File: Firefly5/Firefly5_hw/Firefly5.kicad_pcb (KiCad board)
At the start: 2 copper layers, 63 x 16 mm, 52 parts, among them Q1 LED_5050, Q2 ALS-PT19-315C, SW1 SWITCH, SW2 Btn4x4, SW3 Btn4x4

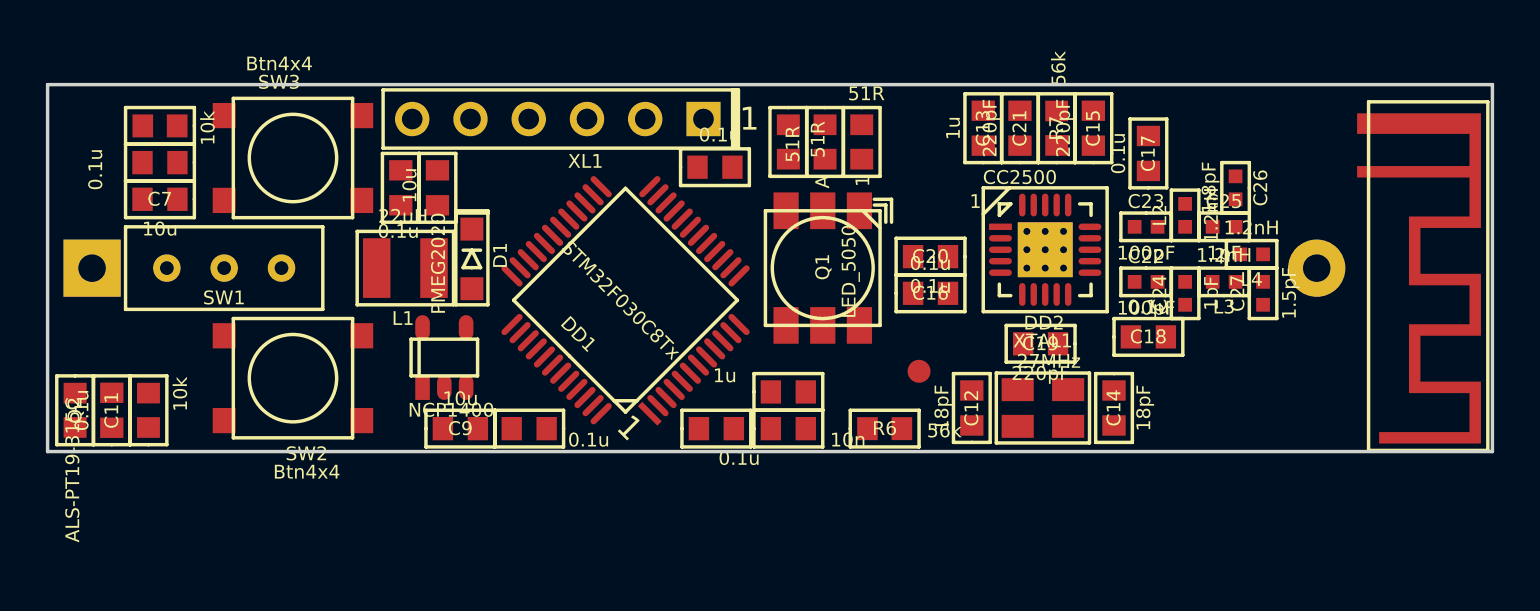
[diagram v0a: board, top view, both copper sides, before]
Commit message: Firefly5 ready for production
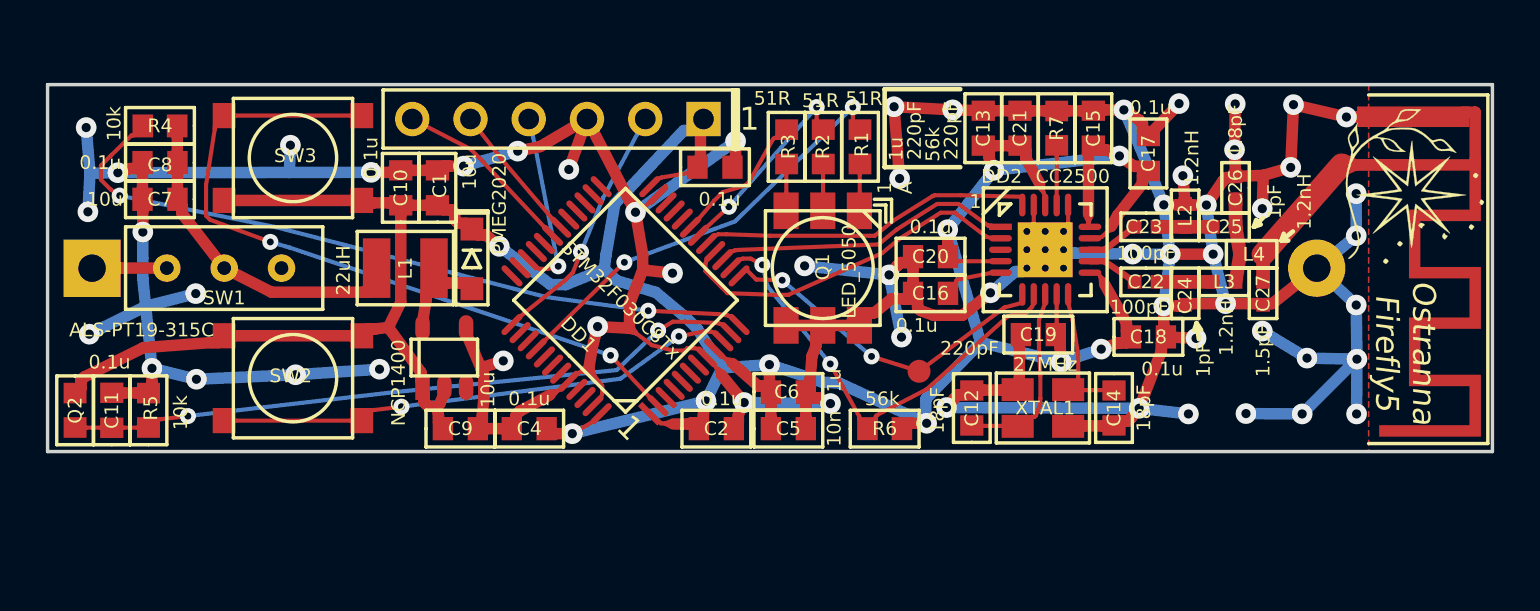
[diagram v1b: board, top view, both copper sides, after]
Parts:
- added Logo1: Logo, Pictures:Ostranna_8x8, F.Cu at (221.8, 99.9)
- moved C19 0.41 mm to (205.6, 106.0)
- moved ANT1 0.30 mm to (220.0, 98.6)
- moved R1 0.22 mm to (197.8, 97.8)
- moved R2 0.22 mm to (196.2, 97.8)
- moved R3 0.22 mm to (194.6, 97.8)
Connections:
- DA1 pad 3: (no net) -> Net-(DA1-Pad3)
- DD1 pad 20: (no net) -> Net-(DD1-Pad20)
- DD1 pad 21: (no net) -> Net-(DD1-Pad21)
- DD1 pad 22: (no net) -> Net-(DD1-Pad22)
- DD1 pad 25: (no net) -> Net-(DD1-Pad25)
- DD1 pad 26: (no net) -> Net-(DD1-Pad26)
- DD1 pad 27: (no net) -> Net-(DD1-Pad27)
- DD1 pad 28: (no net) -> Net-(DD1-Pad28)
- DD1 pad 29: (no net) -> Net-(DD1-Pad29)
- DD1 pad 3: (no net) -> Net-(DD1-Pad3)
- DD1 pad 32: (no net) -> Net-(DD1-Pad32)
- DD1 pad 33: (no net) -> Net-(DD1-Pad33)
- DD1 pad 35: (no net) -> Net-(DD1-Pad35)
- DD1 pad 36: (no net) -> Net-(DD1-Pad36)
- DD1 pad 38: (no net) -> Net-(DD1-Pad38)
- DD1 pad 39: (no net) -> Net-(DD1-Pad39)
- DD1 pad 4: (no net) -> Net-(DD1-Pad4)
- DD1 pad 41: (no net) -> Net-(DD1-Pad41)
- DD1 pad 42: (no net) -> Net-(DD1-Pad42)
- DD1 pad 43: (no net) -> Net-(DD1-Pad43)
- DD1 pad 45: (no net) -> Net-(DD1-Pad45)
- DD1 pad 46: (no net) -> Net-(DD1-Pad46)
- DD1 pad 5: (no net) -> Net-(DD1-Pad5)
- DD1 pad 6: (no net) -> Net-(DD1-Pad6)
- DD1 pad 7: (no net) -> Net-(DD1-Pad7)
- DD2 pad 3: (no net) -> Net-(DD2-Pad3)
- SW1 pad 3: (no net) -> Net-(SW1-Pad3)
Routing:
- net GND: track 0.00 -> 249.7 mm, vias 0 -> 58
- net +3.3V: track 0.00 -> 150.7 mm, vias 0 -> 10
- net /BTN2: track 0.00 -> 32.3 mm, vias 0 -> 2
- net Net-(DD1-Pad12): track 0.00 -> 32.0 mm, vias 0 -> 2
- net /LUM_MEAS: track 0.00 -> 29.8 mm, vias 0 -> 2
- net /BTN1: track 0.00 -> 22.8 mm, vias 0 -> 2
- net /CC_CS: track 0.00 -> 19.9 mm, vias 0 -> 2
- net /BLUE_LED: track 0.00 -> 18.8 mm, vias 0 -> 2
- net /CC_MISO: track 0.00 -> 15.6 mm
- net /CC_GDO0: track 0.00 -> 15.3 mm, vias 0 -> 2
- net /CC_MOSI: track 0.00 -> 14.8 mm
- net +BATT: track 0.00 -> 14.6 mm
- net /CC_SCK: track 0.00 -> 13.1 mm
- net /SWCLK: track 0.00 -> 10.9 mm, vias 0 -> 1
- net Net-(ANT1-Pad1): track 0.00 -> 10.6 mm
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- added copper zone on B.Cu, net GND
- added copper zone on F.Cu, net GND
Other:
- net class Default: trace_width 0.2 -> 0.18; via_dia 0.9 -> 0.7; via_drill 0.4 -> 0.3
- net class Wide: clearance 0.2 -> 0.18
- rule trace_min: 0.2 -> 0.1
- rule via_min_drill: 0.4 -> 0.3
- rule via_min_size: 0.889 -> 0.6
- board text added: "Ostranna Firefly5"

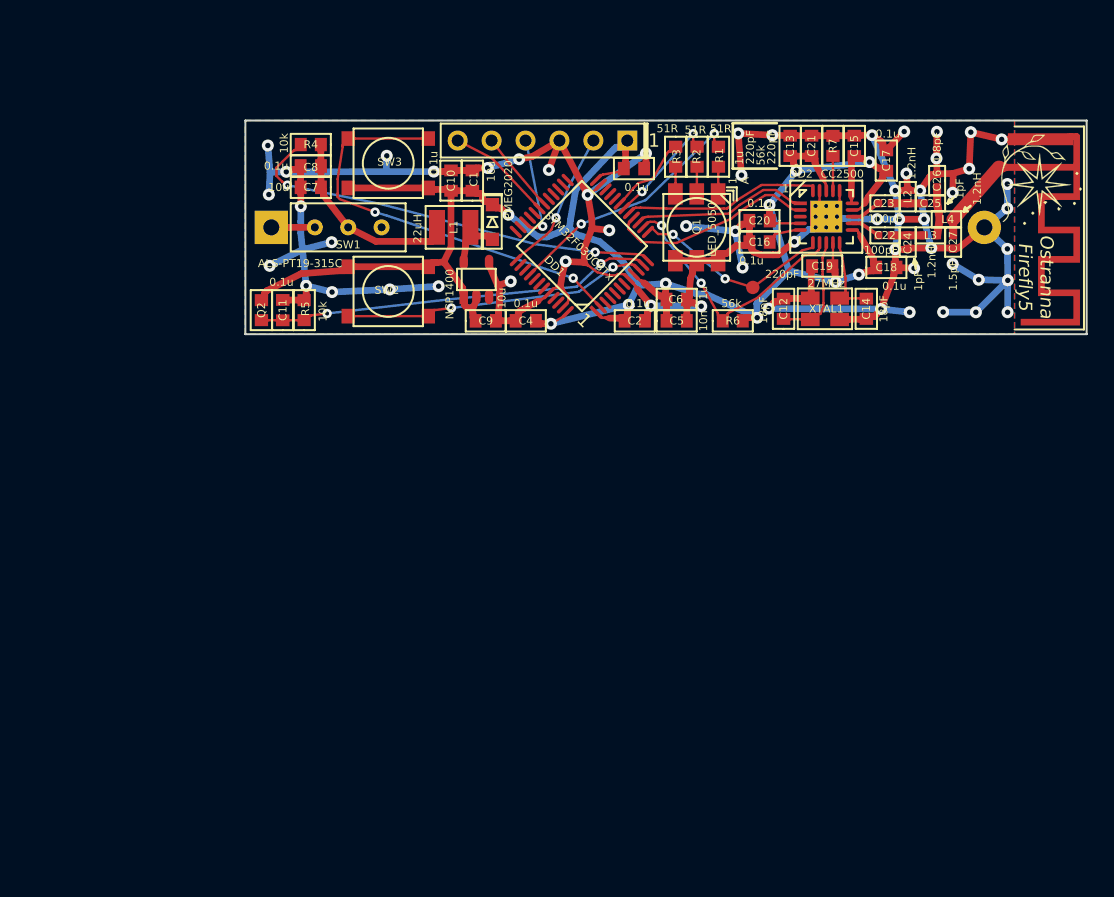
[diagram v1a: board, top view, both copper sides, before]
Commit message: * Something in FF3 + FF5.1
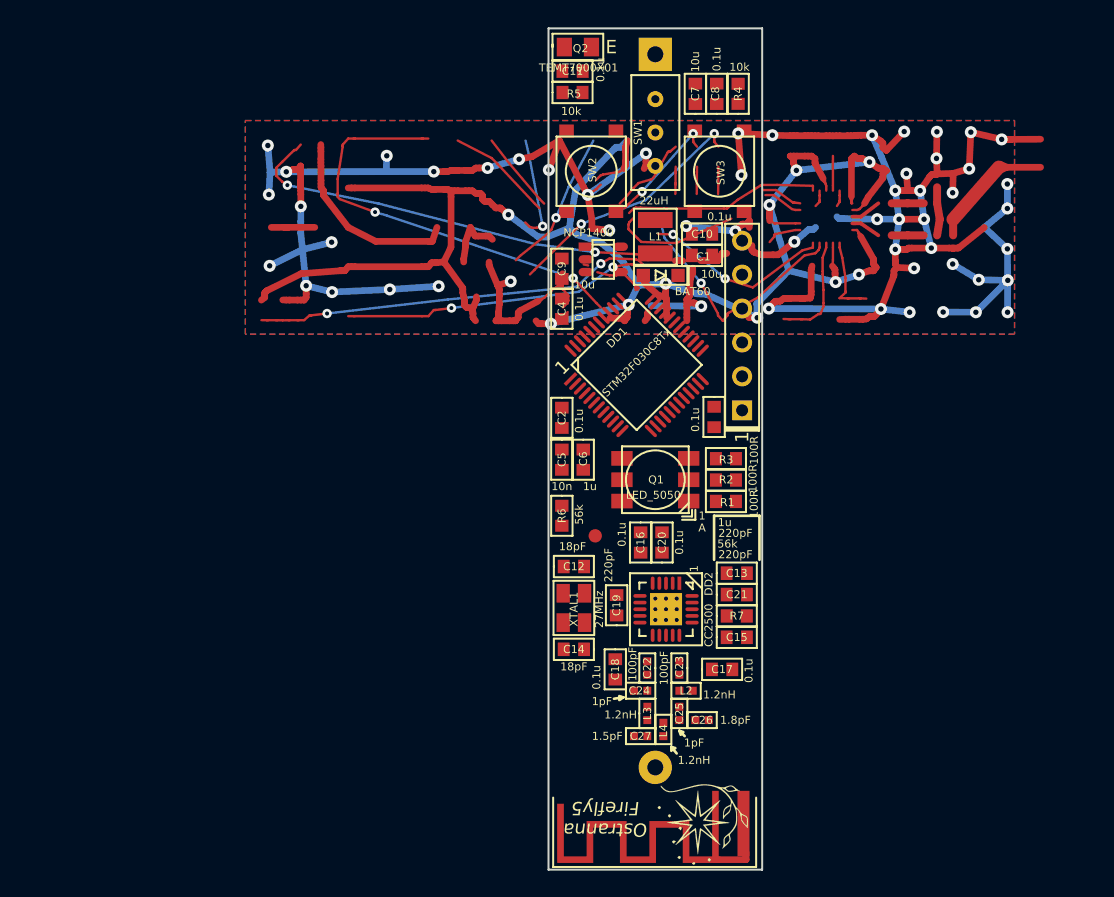
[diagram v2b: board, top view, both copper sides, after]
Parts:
- D1: value PMEG2020 -> BAT60
- Q2: value ALS-PT19-315C -> TEMT7000X01; footprint Resistors:RES_0603 -> Resistors:RES_0805
- R1, R2, R3: value 51R -> 100R
- moved Logo1 54.1 mm to (196.3, 147.6), turned to 180 degrees
- moved ANT1 52.2 mm to (197.6, 145.8), turned to 0 degrees
- moved C26 44.1 mm to (196.6, 140.0), turned to 180 degrees
- moved C27 43.8 mm to (192.0, 141.2), turned to 0 degrees
- moved L4 43.7 mm to (193.7, 140.7), turned to 90 degrees
- moved C25 42.6 mm to (194.9, 139.5), turned to 270 degrees
- moved L3 41.6 mm to (192.5, 139.5), turned to 90 degrees
- moved L2 40.6 mm to (195.4, 137.8), turned to 0 degrees
- moved C17 40.0 mm to (198.1, 136.2), turned to 0 degrees
- moved C24 39.1 mm to (192.0, 137.8), turned to 0 degrees
- moved C23 38.1 mm to (194.9, 136.1), turned to 270 degrees
- moved C15 37.8 mm to (199.2, 133.8), turned to 0 degrees
- moved C22 37.0 mm to (192.5, 136.1), turned to 270 degrees
- moved C18 36.3 mm to (190.1, 136.2), turned to 270 degrees
- moved R7 35.9 mm to (199.2, 132.2), turned to 0 degrees
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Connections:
- DA1 pad 3: Net-(DA1-Pad3) -> (no net)
- DD1 pad 20: Net-(DD1-Pad20) -> (no net)
- DD1 pad 21: Net-(DD1-Pad21) -> (no net)
- DD1 pad 22: Net-(DD1-Pad22) -> (no net)
- DD1 pad 25: Net-(DD1-Pad25) -> (no net)
- DD1 pad 26: Net-(DD1-Pad26) -> (no net)
- DD1 pad 27: Net-(DD1-Pad27) -> (no net)
- DD1 pad 28: Net-(DD1-Pad28) -> (no net)
- DD1 pad 3: Net-(DD1-Pad3) -> (no net)
- DD1 pad 32: Net-(DD1-Pad32) -> (no net)
- DD1 pad 33: Net-(DD1-Pad33) -> (no net)
- DD1 pad 35: Net-(DD1-Pad35) -> (no net)
- DD1 pad 36: Net-(DD1-Pad36) -> (no net)
- DD1 pad 38: Net-(DD1-Pad38) -> (no net)
- DD1 pad 39: Net-(DD1-Pad39) -> (no net)
- DD1 pad 4: Net-(DD1-Pad4) -> (no net)
- DD1 pad 41: Net-(DD1-Pad41) -> (no net)
- DD1 pad 42: Net-(DD1-Pad42) -> (no net)
- DD1 pad 43: Net-(DD1-Pad43) -> (no net)
- DD1 pad 45: Net-(DD1-Pad45) -> (no net)
- DD1 pad 46: Net-(DD1-Pad46) -> (no net)
- DD1 pad 5: Net-(DD1-Pad5) -> (no net)
- DD1 pad 6: Net-(DD1-Pad6) -> (no net)
- DD1 pad 7: Net-(DD1-Pad7) -> (no net)
- DD2 pad 3: Net-(DD2-Pad3) -> (no net)
- Q2 pad 1: +3.3V -> /LUM_MEAS
- Q2 pad 2: /LUM_MEAS -> GND
- R5 pad 1: /LUM_MEAS -> Net-(DD1-Pad29)
- R5 pad 2: GND -> /LUM_MEAS
- SW1 pad 3: Net-(SW1-Pad3) -> (no net)
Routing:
- net GND: track 249.7 -> 156.6 mm, vias 58 -> 27
- net /BTN2: track 32.3 -> 122.2 mm, vias 2 -> 25
- net /Lout: track 4.81 -> 66.6 mm, vias 0 -> 4
- net Net-(DD1-Pad12): track 32.0 -> 0.00 mm, vias 2 -> 0
- net /LUM_MEAS: track 29.8 -> 0.00 mm, vias 2 -> 0
- net /BTN1: track 22.8 -> 0.00 mm, vias 2 -> 0
- net Net-(DD1-Pad21): track 0.00 -> 22.3 mm, vias 0 -> 2
- net Net-(SW1-Pad3): track 0.00 -> 21.5 mm, vias 0 -> 9
- net /CC_GDO0: track 15.3 -> 0.00 mm, vias 2 -> 0
- net /SWCLK: track 10.9 -> 0.00 mm, vias 1 -> 0
- net /CC_SCK: track 13.1 -> 3.08 mm
- net +3.3V: track 150.7 -> 159.4 mm, vias 10 -> 12
- net /RED_LED: track 8.69 -> 0.00 mm, vias 2 -> 0
- net /SWDIO: track 8.02 -> 0.00 mm, vias 1 -> 0
- net Net-(DD1-Pad45): track 0.00 -> 6.39 mm
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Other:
- board size 63 x 16 mm -> 16 x 63 mm
- net class Default: trace_width 0.18 -> 0.25
- board text added: "E"

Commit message: Firefly 5.1 sent to factory
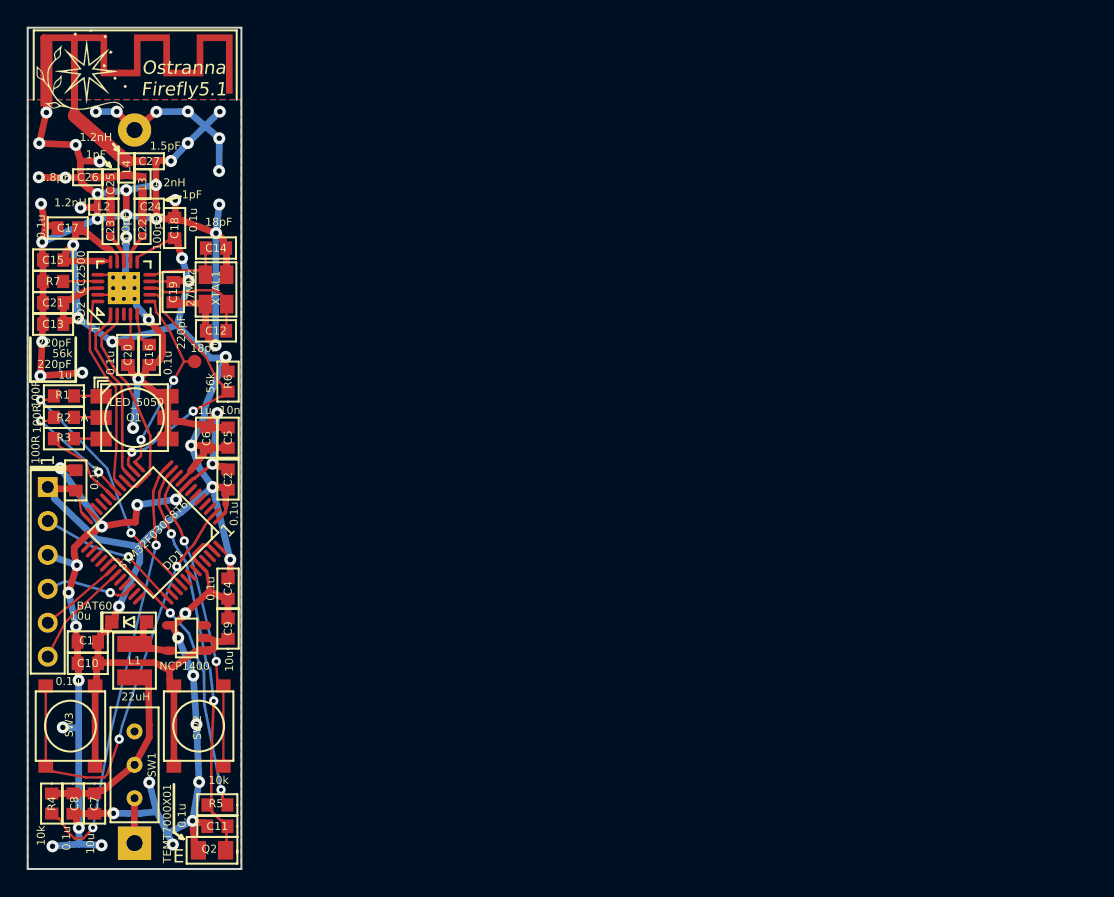
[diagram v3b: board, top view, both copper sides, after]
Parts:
- DD1: value STM32F030C8Tx -> STM32F030C8T6
- moved R4 73.9 mm to (147.9, 146.2), turned to 270 degrees
- moved Logo1 72.4 mm to (150.5, 91.5), turned to 0 degrees
- moved C8 71.8 mm to (149.5, 146.2), turned to 270 degrees
- moved ANT1 71.0 mm to (149.6, 93.5), turned to 180 degrees
- moved C7 69.6 mm to (151.1, 146.2), turned to 270 degrees
- moved Q2 66.1 mm to (159.9, 149.8), turned to 180 degrees
- moved SW3 63.9 mm to (149.3, 140.4), turned to 270 degrees
- moved C11 62.5 mm to (160.3, 147.9), turned to 180 degrees
- moved C26 61.4 mm to (150.6, 99.3), turned to 0 degrees
- moved SW1 61.3 mm to (154.1, 143.3), turned to 90 degrees
- moved R5 59.6 mm to (160.3, 146.3), turned to 180 degrees
- moved C17 59.1 mm to (149.1, 103.2), turned to 180 degrees
- moved C15 58.5 mm to (148.0, 105.5), turned to 180 degrees
- moved C25 58.2 mm to (152.3, 99.8), turned to 90 degrees
- moved L4 58.2 mm to (153.5, 98.7), turned to 270 degrees
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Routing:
- net /BTN2: track 122.2 -> 32.2 mm, vias 25 -> 2
- net GND: track 156.6 -> 236.5 mm, vias 27 -> 58
- net /Lout: track 66.6 -> 4.81 mm, vias 4 -> 0
- net Net-(DD1-Pad12): track 0.00 -> 32.2 mm, vias 0 -> 2
- net /LUM_MEAS: track 0.00 -> 30.2 mm, vias 0 -> 2
- net /BTN1: track 0.00 -> 22.9 mm, vias 0 -> 2
- net Net-(DD1-Pad21): track 22.3 -> 0.00 mm, vias 2 -> 0
- net Net-(DD1-Pad29): track 0.00 -> 22.1 mm, vias 0 -> 2
- net Net-(SW1-Pad3): track 21.5 -> 0.00 mm, vias 9 -> 0
- net +3.3V: track 159.4 -> 141.3 mm, vias 12 -> 10
- net /CC_GDO0: track 0.00 -> 15.2 mm, vias 0 -> 2
- net /SWCLK: track 0.00 -> 10.9 mm, vias 0 -> 1
- net /CC_SCK: track 3.08 -> 13.4 mm
- net /RED_LED: track 0.00 -> 8.69 mm, vias 0 -> 2
- net /SWDIO: track 0.00 -> 6.57 mm, vias 0 -> 1
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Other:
- board text added: "Ostranna Firefly5.1"
- board text removed: "Ostranna Firefly5"
